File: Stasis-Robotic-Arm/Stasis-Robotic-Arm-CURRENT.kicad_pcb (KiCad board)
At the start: 2 copper layers, 122.5 x 79.5 mm, 81 parts, among them J1 Screw_Terminal_01x04, J2 USB_C_Receptacle_USB2.0_14P, J3 Screw_Terminal_01x04, J4 Screw_Terminal_01x04, J5 Screw_Terminal_01x04, J6 Screw_Terminal_01x04, J7 Screw_Terminal_01x02, J8 Screw_Terminal_01x03, SW1 Enable, SW2 boot, U10 TVS1400DRV, U4 NCP1117-3.3_SOT223, U8 NCP1117-3.3_SOT223, U9 TVS1400DRV

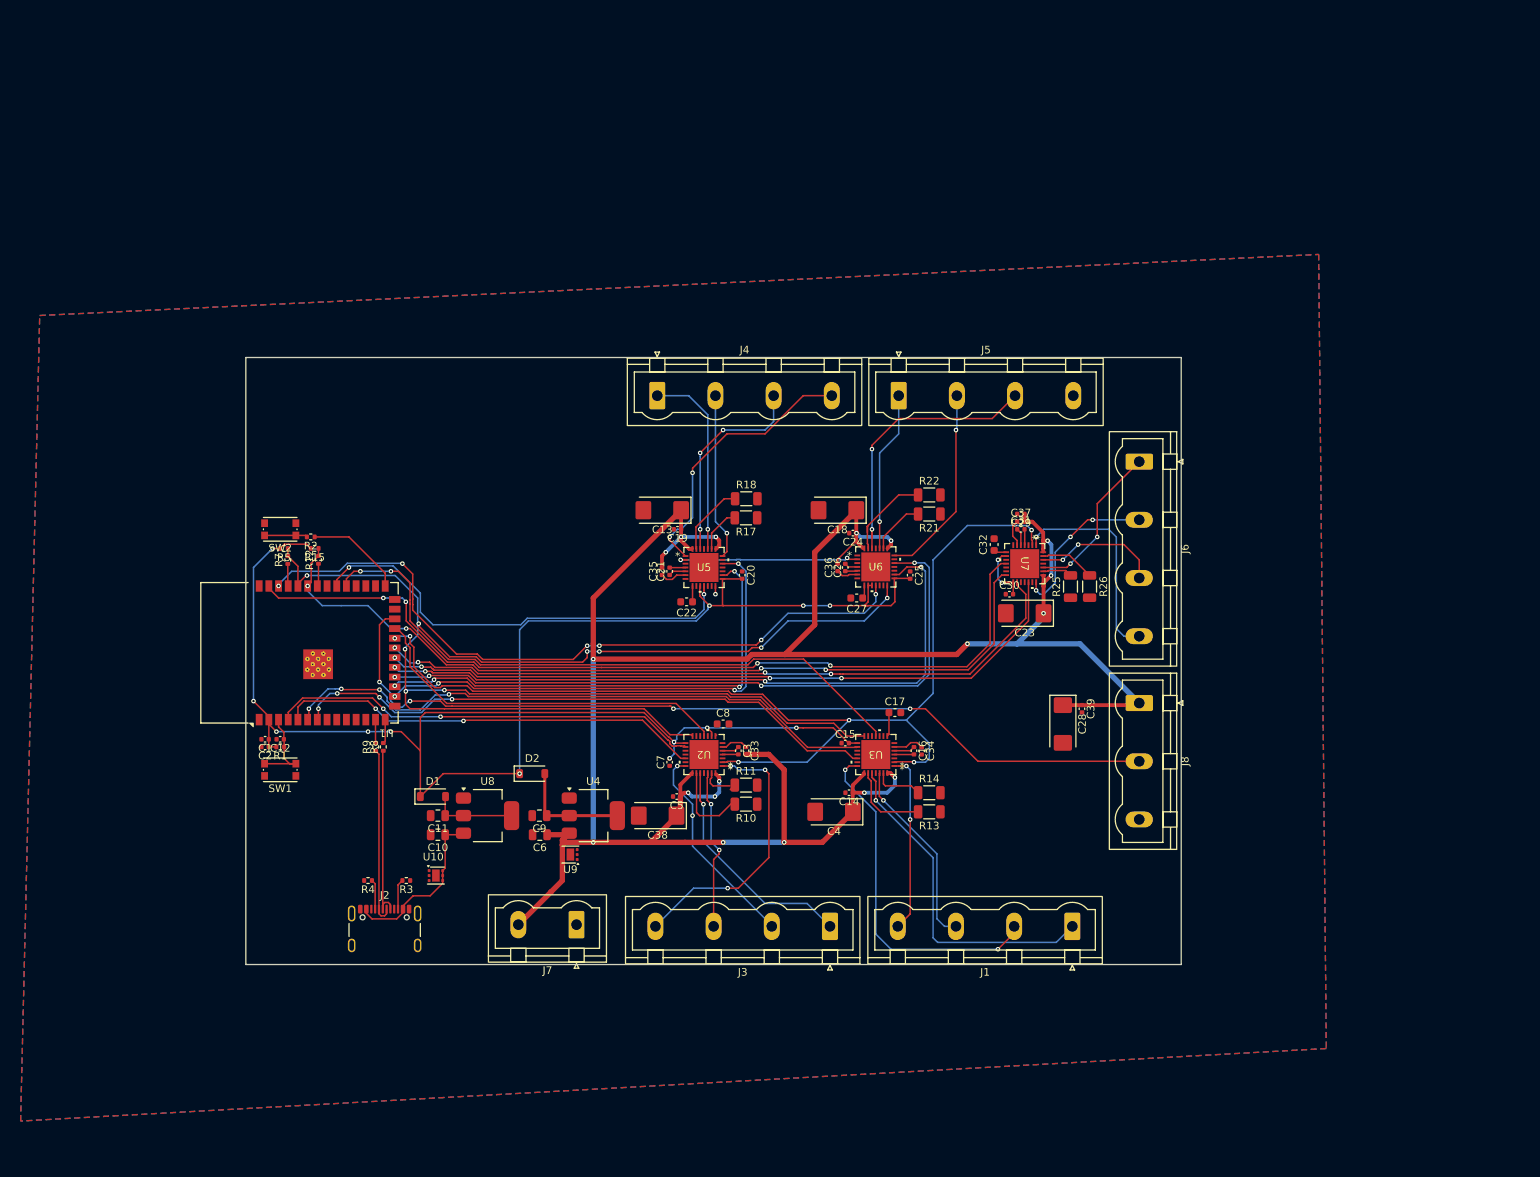
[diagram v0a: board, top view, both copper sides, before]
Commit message: Add files via upload
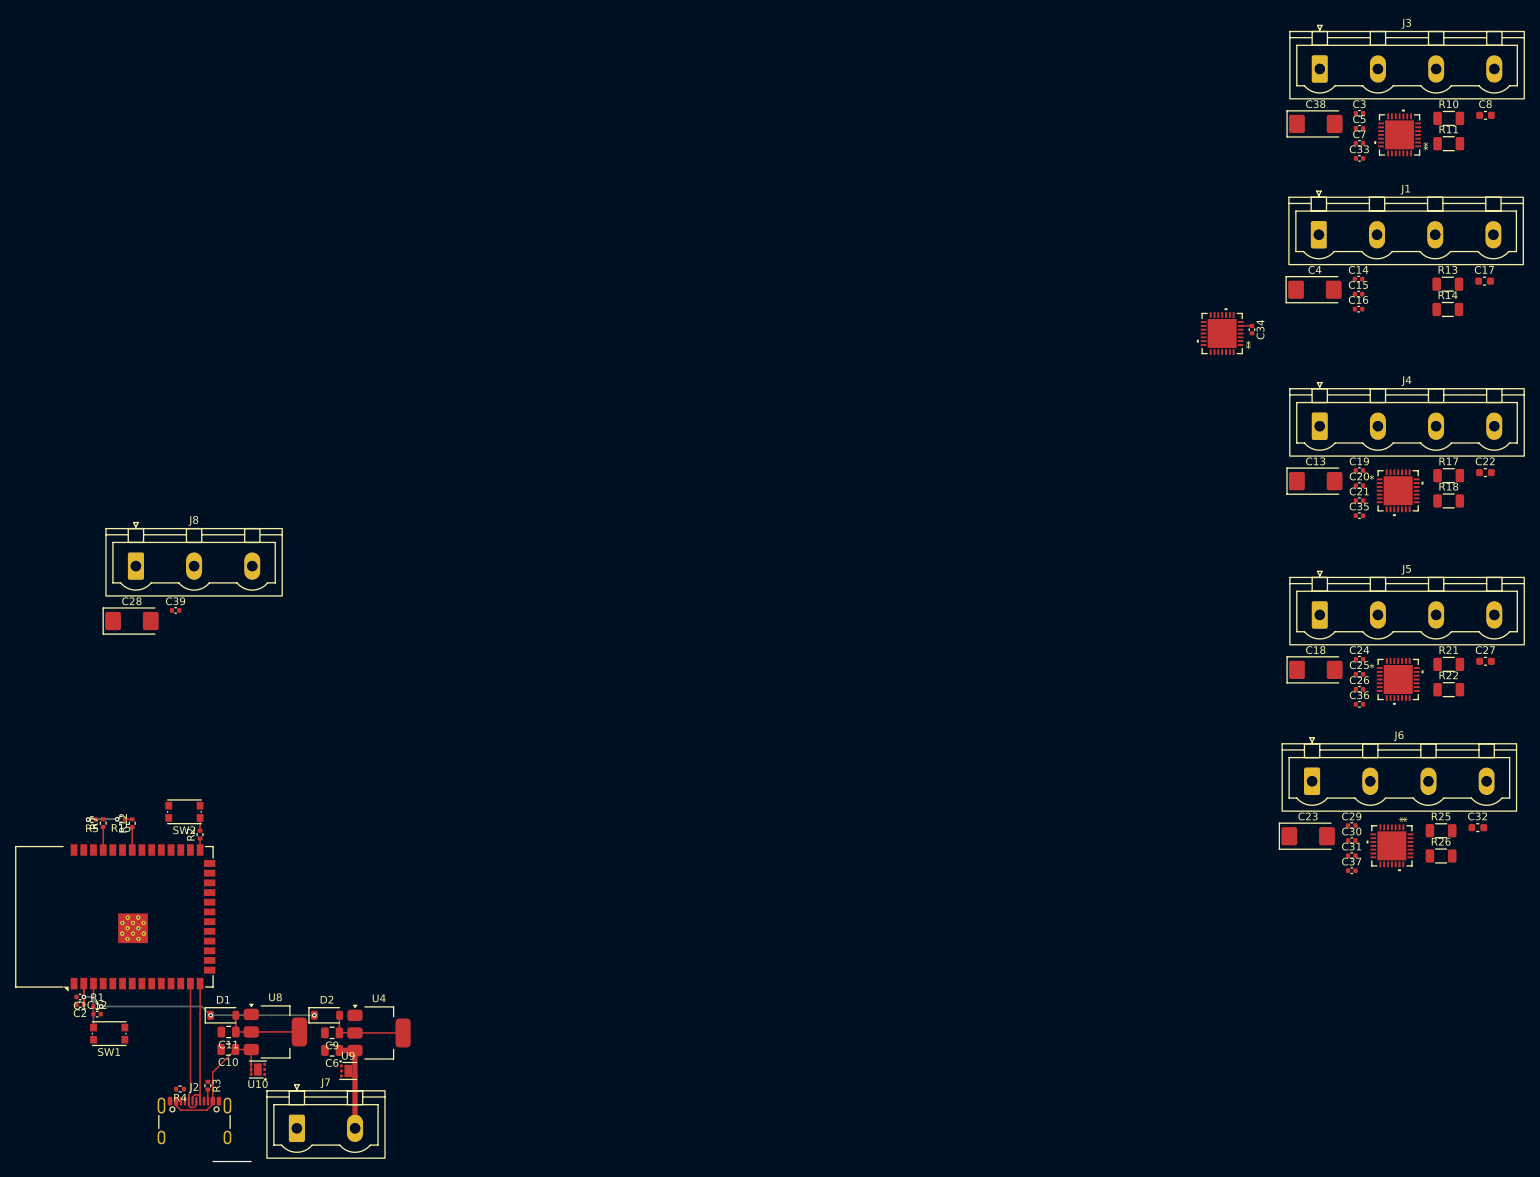
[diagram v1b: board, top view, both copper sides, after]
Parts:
- removed R8, R9: 22, Resistor_SMD:R_0402_1005Metric
- moved J8 132.6 mm to (53.1, 84.8), turned to 0 degrees
- moved J3 129.3 mm to (208.1, 19.7), turned to 0 degrees
- moved R10 128.6 mm to (225.0, 26.2), turned to 0 degrees
- moved C8 127.8 mm to (229.8, 25.8)
- moved C5 125.1 mm to (213.3, 27.5), turned to 0 degrees
- moved C38 125.0 mm to (207.6, 26.9), turned to 0 degrees
- moved R11 124.6 mm to (225.0, 29.5)
- moved C28 122.7 mm to (52.6, 92.0), turned to 0 degrees
- moved U2 122.0 mm to (218.6, 28.3)
- moved C7 121.4 mm to (213.3, 29.5), turned to 0 degrees
- moved C39 119.4 mm to (58.3, 90.6), turned to 0 degrees
- moved C3 116.6 mm to (213.3, 25.5), turned to 0 degrees
- moved C33 111.7 mm to (213.3, 31.4), turned to 0 degrees
- moved C22 106.0 mm to (229.8, 72.6), turned to 0 degrees
- moved R13 96.9 mm to (224.9, 47.9), turned to 0 degrees
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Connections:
- C25 pad 2: +3V3 -> Net-(U6-VCC_IO)
- J2 pad A6: Net-(J2-D+-PadA6) -> /D+
- J2 pad A7: Net-(J2-D--PadA7) -> /D-
- J2 pad B6: Net-(J2-D+-PadA6) -> /D+
- J2 pad B7: Net-(J2-D--PadA7) -> /D-
- U6 pad 15: +3V3 -> Net-(U6-VCC_IO)
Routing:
- net VBAT: track 321.0 -> 12.2 mm, vias 18 -> 0
- net /PDN-UART0: track 210.0 -> 0.00 mm, vias 10 -> 0
- net +3V3: track 243.1 -> 44.5 mm, vias 15 -> 6
- net /ENN: track 167.4 -> 0.00 mm, vias 8 -> 0
- net /PWM: track 114.9 -> 0.00 mm, vias 4 -> 0
- net /DIAG_5: track 114.0 -> 0.00 mm, vias 4 -> 0
- net /PDN-UART1: track 112.6 -> 0.96 mm, vias 4 -> 0
- net /DIAG_4: track 92.8 -> 0.00 mm, vias 6 -> 0
- net /STEP_5: track 92.7 -> 0.00 mm, vias 4 -> 0
- net /DIR_5: track 92.1 -> 0.00 mm, vias 4 -> 0
- net /DIR_4: track 90.3 -> 0.00 mm, vias 4 -> 0
- net /STEP_4: track 89.2 -> 0.00 mm, vias 4 -> 0
- net /DIAG_2: track 83.5 -> 0.00 mm, vias 2 -> 0
- net /STEP_2: track 79.7 -> 0.00 mm, vias 4 -> 0
- net /DIR_2: track 78.1 -> 0.00 mm, vias 4 -> 0
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- removed copper zone on B.Cu, net GND
- removed copper zone on F.Cu, net GND
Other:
- board outline removed

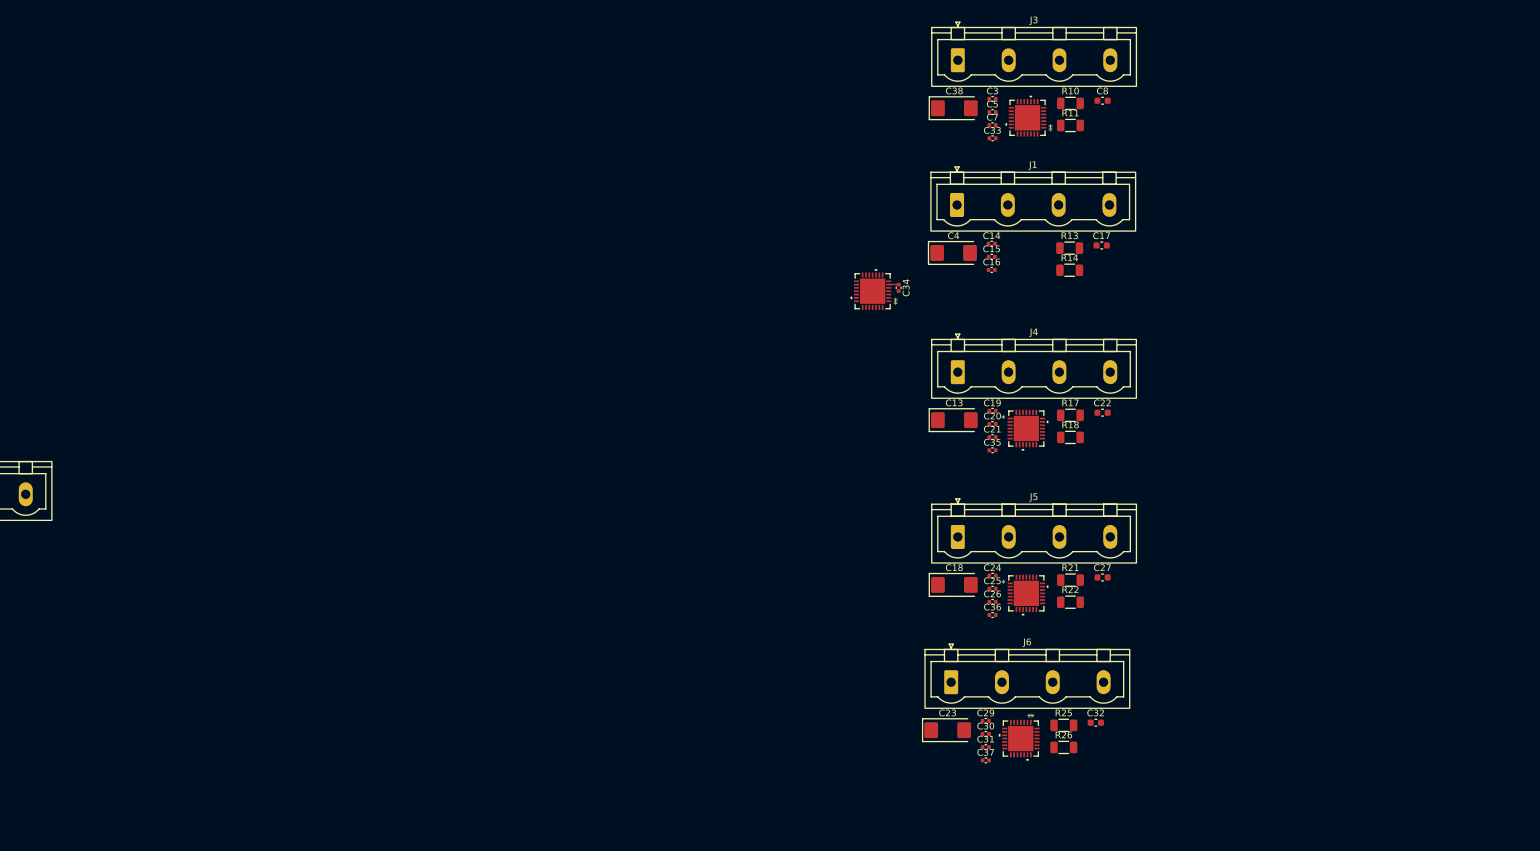
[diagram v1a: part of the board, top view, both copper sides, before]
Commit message: Add files via upload
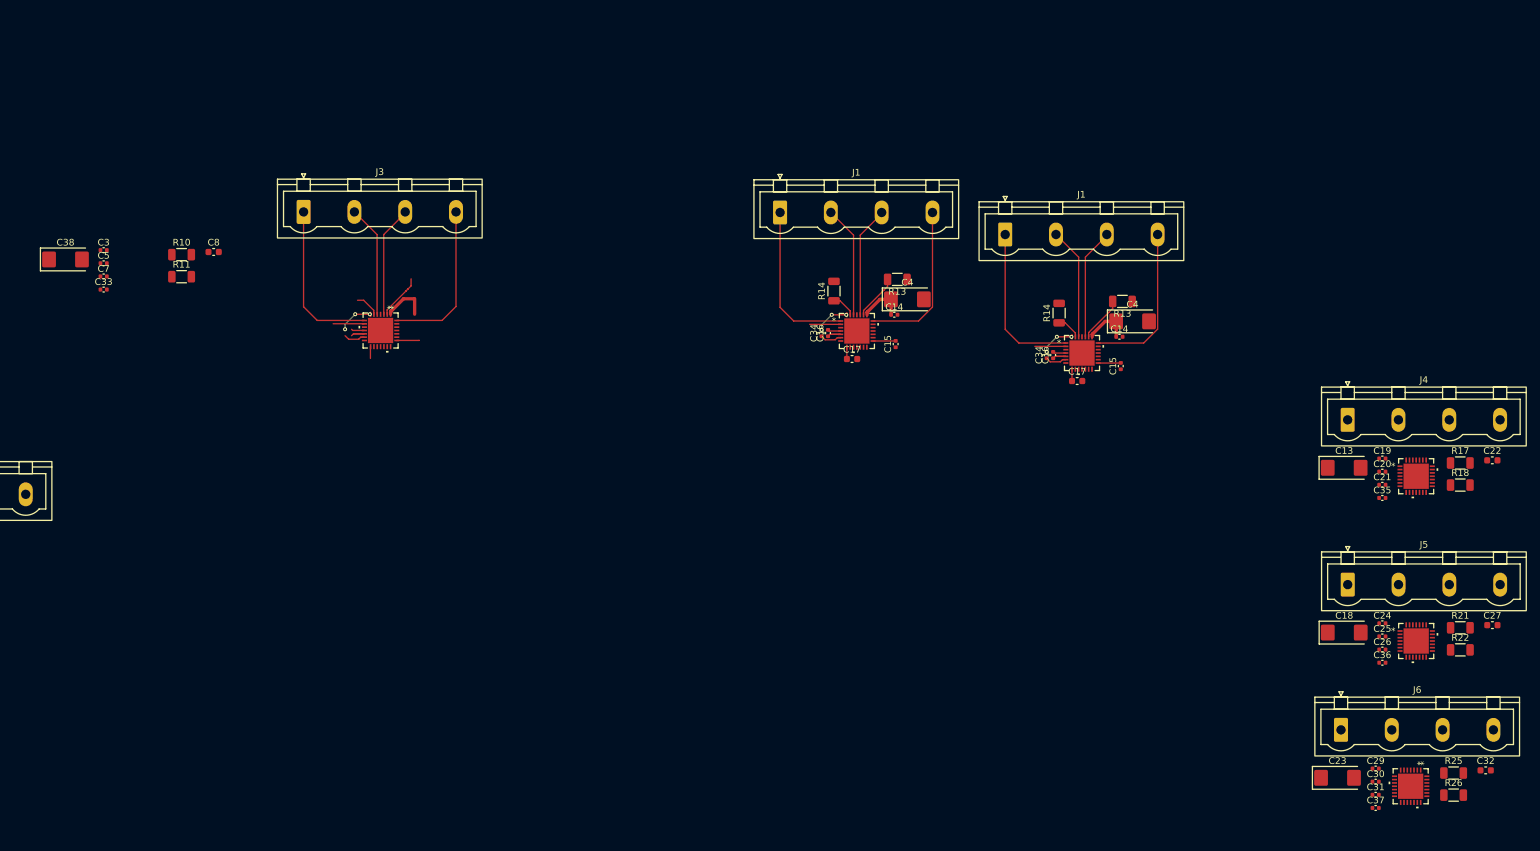
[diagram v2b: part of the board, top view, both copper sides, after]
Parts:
- added C14: 100nF, Capacitor_SMD:C_0402_1005Metric, F.Cu at (232.4, 61.2)
- added C15: 100nF, Capacitor_SMD:C_0402_1005Metric, F.Cu at (232.6, 65.6)
- added C16: 22nF, Capacitor_SMD:C_0402_1005Metric, F.Cu at (222.4, 63.9)
- added C17: 2.2μF, Capacitor_SMD:C_0603_1608Metric, F.Cu at (226.0, 67.8)
- added C34: 100nF, Capacitor_SMD:C_0402_1005Metric, F.Cu at (221.5, 63.9)
- added C4: 100μF, Capacitor_Tantalum_SMD:CP_EIA-6032-28_Kemet-C, F.Cu at (234.3, 58.9)
- added J1: Screw_Terminal_01x04, Connector_Phoenix_GMSTB:PhoenixContact_GMSTBVA_2,5_4-G-7,62_1x04_P7.62mm_Vertical, F.Cu at (215.2, 45.9)
- added R13: 0.1, Resistor_SMD:R_1206_3216Metric, F.Cu at (232.8, 55.9)
- added R14: 0.1, Resistor_SMD:R_1206_3216Metric, F.Cu at (223.3, 57.6)
- added U3: ~, MyFootprintLibrary:tmc2209, F.Cu at (226.8, 63.6)
- moved C3 135.2 mm to (80.0, 48.2)
- moved C33 135.2 mm to (80.0, 54.1)
- moved C38 135.2 mm to (74.3, 49.6)
- moved C5 135.2 mm to (80.0, 50.2)
- moved C7 135.2 mm to (80.0, 52.1)
- moved C8 135.2 mm to (96.5, 48.5)
- moved R10 135.2 mm to (91.7, 48.9)
- moved R11 135.2 mm to (91.7, 52.2)
- moved U2 102.1 mm to (121.6, 60.2), turned to -90 degrees
- moved J3 100.7 mm to (110.0, 42.5)
- moved C18 58.9 mm to (266.1, 105.6)
- moved J4 58.9 mm to (266.6, 73.7)
- moved J6 58.9 mm to (265.6, 120.2)
- moved U6 58.9 mm to (276.9, 106.8)
- moved U7 58.9 mm to (276.1, 128.6)
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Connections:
- U2 pad 1: Net-(J3-Pin_4) -> Net-(J3-Pin_1)
- U2 pad 21: Net-(J3-Pin_2) -> Net-(J3-Pin_4)
- U2 pad 24: Net-(J3-Pin_1) -> Net-(J3-Pin_3)
- U2 pad 26: Net-(J3-Pin_3) -> Net-(J3-Pin_2)
- U3 pad 1: Net-(J1-Pin_4) -> Net-(J1-Pin_1)
- U3 pad 21: Net-(J1-Pin_2) -> Net-(J1-Pin_4)
- U3 pad 24: Net-(J1-Pin_1) -> Net-(J1-Pin_3)
- U3 pad 26: Net-(J1-Pin_3) -> Net-(J1-Pin_2)
- U5 pad 1: Net-(J4-Pin_4) -> Net-(J4-Pin_1)
- U5 pad 21: Net-(J4-Pin_2) -> Net-(J4-Pin_4)
- U5 pad 24: Net-(J4-Pin_1) -> Net-(J4-Pin_3)
- U5 pad 26: Net-(J4-Pin_3) -> Net-(J4-Pin_2)
- U6 pad 1: Net-(J5-Pin_4) -> Net-(J5-Pin_1)
- U6 pad 21: Net-(J5-Pin_2) -> Net-(J5-Pin_4)
- U6 pad 24: Net-(J5-Pin_1) -> Net-(J5-Pin_3)
- U6 pad 26: Net-(J5-Pin_3) -> Net-(J5-Pin_2)
- U7 pad 1: Net-(J6-Pin_4) -> Net-(J6-Pin_1)
- U7 pad 21: Net-(J6-Pin_2) -> Net-(J6-Pin_4)
- U7 pad 24: Net-(J6-Pin_1) -> Net-(J6-Pin_3)
- U7 pad 26: Net-(J6-Pin_3) -> Net-(J6-Pin_2)
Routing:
- net Net-(J1-Pin_1): track 0.00 -> 48.6 mm
- net Net-(J1-Pin_4): track 0.00 -> 47.9 mm
- net Net-(J1-Pin_3): track 0.00 -> 35.0 mm
- net Net-(J1-Pin_2): track 0.00 -> 33.5 mm
- net Net-(J3-Pin_1): track 0.00 -> 31.4 mm
- net VBAT: track 12.2 -> 40.2 mm, vias 0 -> 6
- net Net-(J3-Pin_4): track 0.00 -> 24.0 mm
- net Net-(J3-Pin_3): track 0.00 -> 17.5 mm
- net Net-(J3-Pin_2): track 0.00 -> 16.8 mm
- net /ENN: track 0.00 -> 16.1 mm
- net Net-(U3-BRA): track 0.00 -> 13.6 mm
- net +3V3: track 44.5 -> 57.7 mm
- net Net-(U3-BRB): track 0.00 -> 7.29 mm
- net Net-(U3-CPI): track 0.00 -> 7.08 mm
- net unconnected-(U2-SPREAD-Pad7): track 0.00 -> 5.17 mm, vias 0 -> 3
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
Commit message: Add files via upload
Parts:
- removed the C14 at (232.4, 61.2)
- removed the C14 at (198.6, 57.9)
- removed the C15 at (232.6, 65.6)
- removed the C15 at (198.8, 62.3)
- removed the C16 at (222.4, 63.9)
- removed the C16 at (188.7, 60.6)
- removed the C17 at (226.0, 67.8)
- removed the C17 at (192.3, 64.5)
- removed the C34 at (221.5, 63.9)
- removed the C34 at (187.7, 60.6)
- removed the C4 at (234.3, 58.9)
- removed the C4 at (200.6, 55.6)
- removed the J1 at (181.5, 42.5)
- removed the J1 at (215.2, 45.9)
- removed the R13 at (199.1, 52.6)
- removed the R13 at (232.8, 55.9)
- removed the R14 at (223.3, 57.6)
- removed the R14 at (189.6, 54.3)
- removed the U3 at (226.8, 63.6)
- removed the U3 at (193.0, 60.3)
- added C14: 100nF, Capacitor_SMD:C_0402_1005Metric, F.Cu at (134.2, 147.8)
- added C15: 100nF, Capacitor_SMD:C_0402_1005Metric, F.Cu at (135.3, 143.4)
- added C16: 22nF, Capacitor_SMD:C_0402_1005Metric, F.Cu at (143.2, 145.1)
- added C17: 2.2μF, Capacitor_SMD:C_0603_1608Metric, F.Cu at (141.1, 141.5)
- added C34: 100nF, Capacitor_SMD:C_0402_1005Metric, F.Cu at (144.1, 145.1)
- added C4: 100μF, Capacitor_Tantalum_SMD:CP_EIA-6032-28_Kemet-C, F.Cu at (131.2, 150.1)
- added J1: Screw_Terminal_01x04, Connector_Phoenix_GMSTB:PhoenixContact_GMSTBVA_2,5_4-G-7,62_1x04_P7.62mm_Vertical, F.Cu at (149.8, 157.4)
- added R13: 0.1, Resistor_SMD:R_1206_3216Metric, F.Cu at (137.1, 150.8)
- added R14: 0.1, Resistor_SMD:R_1206_3216Metric, F.Cu at (140.7, 150.8)
- added U3: ~, MyFootprintLibrary:tmc2209, F.Cu at (138.8, 145.4)
- moved C32 182.9 mm to (104.4, 124.8), turned to 180 degrees
- moved R26 178.2 mm to (104.9, 115.2), turned to 90 degrees
- moved R25 174.5 mm to (108.4, 115.2), turned to -90 degrees
- moved J6 170.6 mm to (95.4, 108.6)
- moved U7 169.5 mm to (106.7, 120.8), turned to 0 degrees
- moved C37 169.2 mm to (102.0, 121.1), turned to 90 degrees
- moved C31 168.1 mm to (102.9, 121.1), turned to 90 degrees
- moved C30 160.6 mm to (110.3, 122.8), turned to 90 degrees
- moved C29 158.6 mm to (112.4, 118.2)
- moved C27 153.5 mm to (136.1, 124.9), turned to 180 degrees
- moved C23 151.1 mm to (114.4, 115.9)
- moved C22 149.3 mm to (148.0, 130.7), turned to 90 degrees
- moved R22 147.0 mm to (136.6, 115.2), turned to 90 degrees
- moved R21 143.7 mm to (140.2, 115.2), turned to -90 degrees
- moved J5 140.0 mm to (127.0, 108.6)
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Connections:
- C25 pad 2: Net-(U6-VCC_IO) -> +3V3
- U1 pad 15: unconnected-(U1-IO3-Pad15) -> /DIR_1
- U1 pad 16: /DIR_3 -> /STEP_1
- U1 pad 17: /STEP_3 -> /DIR_2
- U1 pad 18: /DIR_4 -> /STEP_2
- U1 pad 19: /STEP_4 -> /DIR_3
- U1 pad 20: /DIR_5 -> /STEP_3
- U1 pad 21: /STEP_5 -> /DIR_4
- U1 pad 22: /ENN -> /STEP_4
- U1 pad 23: /DIAG_1 -> /DIR_5
- U1 pad 24: /PWM -> /STEP_5
- U1 pad 25: unconnected-(U1-IO48-Pad25) -> /PWM
- U1 pad 30: unconnected-(U1-IO37-Pad30) -> /DIAG_1
- U1 pad 33: unconnected-(U1-IO40-Pad33) -> /DIAG_4
- U1 pad 34: /TXD1 -> /DIAG_5
- U1 pad 35: /PDN-UART1 -> /TXD1
- U1 pad 38: /DIAG_4 -> /PDN-UART1
- U1 pad 39: /DIAG_5 -> unconnected-(U1-IO1-Pad39)
- U1 pad 4: /STEP_1 -> unconnected-(U1-IO4-Pad4)
- U1 pad 5: /DIR_1 -> unconnected-(U1-IO5-Pad5)
- U1 pad 6: /STEP_2 -> unconnected-(U1-IO6-Pad6)
- U1 pad 7: /DIR_2 -> unconnected-(U1-IO7-Pad7)
- U6 pad 15: Net-(U6-VCC_IO) -> +3V3
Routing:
- net VBAT: track 40.2 -> 315.5 mm, vias 6 -> 15
- net /DIR_3: track 0.00 -> 95.7 mm
- net /DIR_4: track 0.00 -> 95.1 mm
- net /STEP_3: track 0.00 -> 93.4 mm
- net /STEP_4: track 0.00 -> 90.8 mm
- net /DIR_2: track 0.00 -> 78.1 mm
- net /STEP_2: track 0.00 -> 78.0 mm
- net /DIR_5: track 0.00 -> 61.9 mm
- net /STEP_5: track 0.00 -> 57.5 mm
- net /DIR_1: track 0.00 -> 47.5 mm
- net /STEP_1: track 0.00 -> 47.4 mm
- net /ENN: track 16.1 -> 60.2 mm, vias 0 -> 9
- net /PWM: track 0.00 -> 37.2 mm
- net Net-(J1-Pin_1): track 48.6 -> 14.8 mm
- net Net-(J1-Pin_4): track 47.9 -> 16.6 mm
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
